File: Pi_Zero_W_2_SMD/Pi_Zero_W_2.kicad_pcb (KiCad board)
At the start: 2 copper layers, 96.5 x 59.3 mm, 44 parts, among them J1 String1, J2 String2, J3 Power In Right, J4 DMX Out, J5 VIN Voltage, J6 OLED Conn, Q1 DMP3056L, SW1 Down BTN, SW2 Enter BTN, U1 Universe5V, U2 24LC256, U3 Raspberry Pi Zero, U4 74AHCT1G125, U5 74AHCT1G125, U6 SP485CN

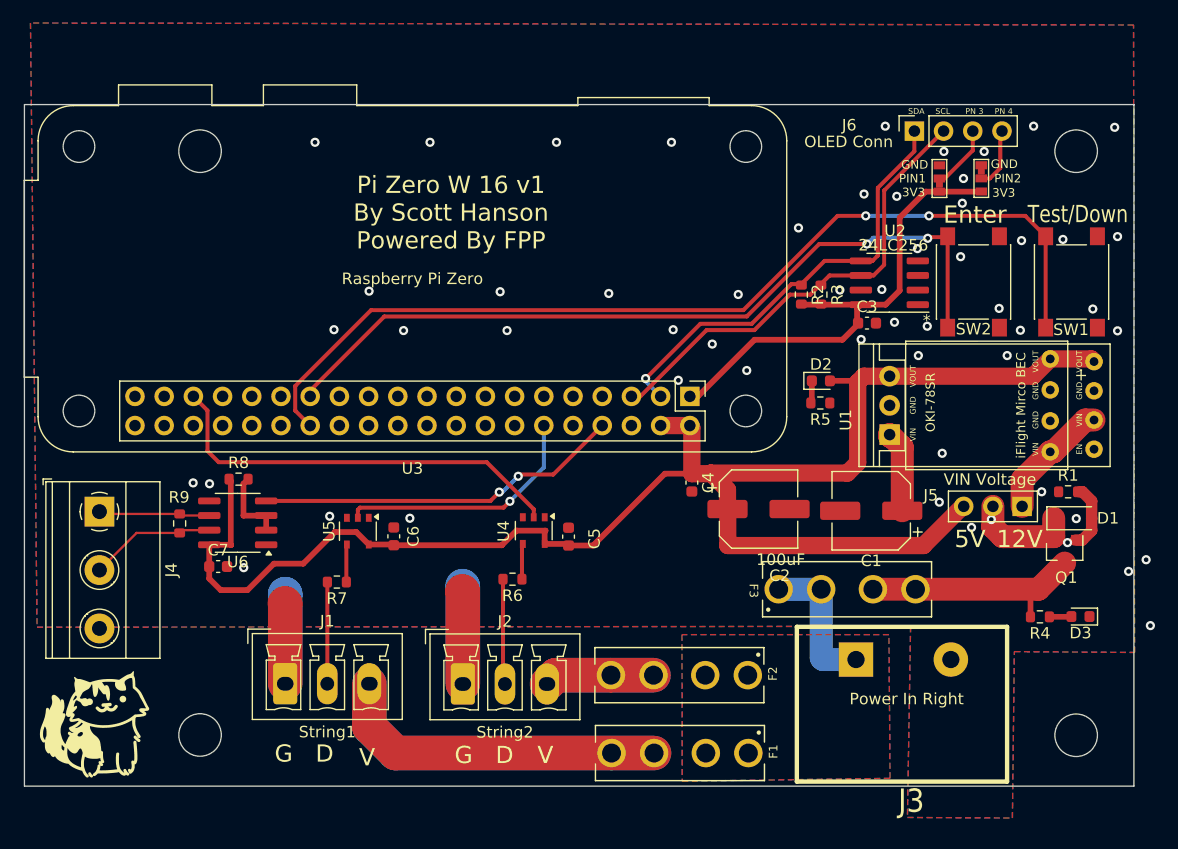
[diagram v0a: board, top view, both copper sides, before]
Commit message: updates
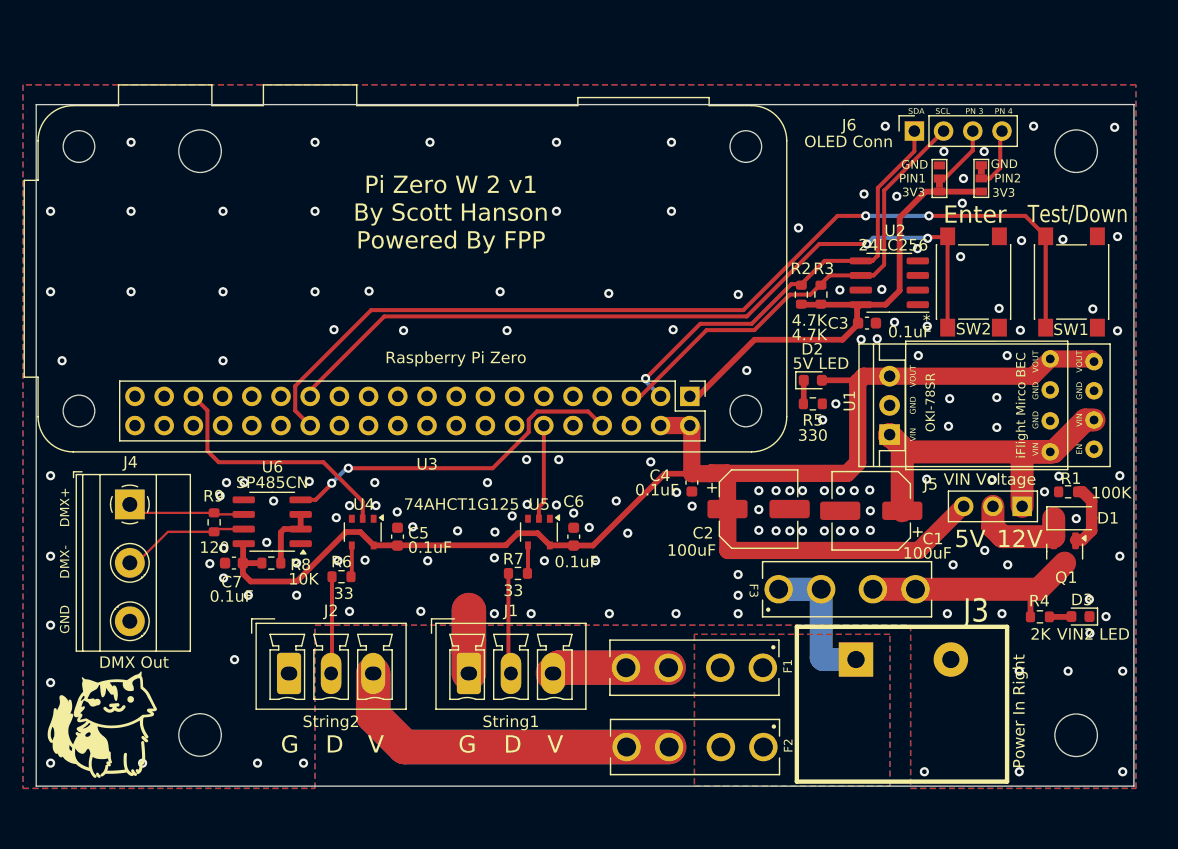
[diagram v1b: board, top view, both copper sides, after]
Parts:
- moved J1 16.0 mm to (156.2, 109.4)
- moved R7 15.8 mm to (160.6, 100.7)
- moved U5 15.8 mm to (162.5, 97.1)
- moved C6 15.7 mm to (165.5, 97.5)
- moved J2 15.1 mm to (140.6, 109.4)
- moved R6 14.9 mm to (145.3, 101.0)
- moved U4 14.9 mm to (147.1, 97.1)
- moved C5 14.9 mm to (150.2, 97.5)
- moved R8 7.84 mm to (139.2, 99.8)
- moved F1 7.53 mm to (176.0, 108.9)
- moved F2 6.40 mm to (176.0, 115.8)
- moved R9 3.00 mm to (134.2, 96.3)
- moved U6 3.00 mm to (139.3, 96.2)
- moved J4 2.72 mm to (126.9, 94.7)
- moved C7 1.41 mm to (135.9, 99.8), turned to 180 degrees
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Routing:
- net /Outputs/VOUT2: track 19.2 -> 61.1 mm
- net /Outputs/VOUT1: track 58.9 -> 20.5 mm
- net GND: track 31.4 -> 11.0 mm, vias 56 -> 155
- net /VIN_Reg: track 18.0 -> 32.5 mm
- net DATA2: track 36.4 -> 22.1 mm
- net DATA1: track 22.0 -> 8.28 mm, vias 1 -> 0
- net +5V: track 141.5 -> 133.0 mm
- net TXD: track 31.9 -> 30.6 mm
- net Net-(R7-Pad1): track 3.29 -> 2.46 mm
- net Net-(U6-DE): track 6.59 -> 5.80 mm
- net /Outputs/DOUT2: track 9.19 -> 8.45 mm
- net /Outputs/DMX+: track 9.69 -> 10.3 mm
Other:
- board size 96.5 x 59.3 mm -> 95.5 x 59.3 mm
- board text added: "DMX+"
- board text added: "DMX-"
